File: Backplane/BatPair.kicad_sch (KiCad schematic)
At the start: 6 parts

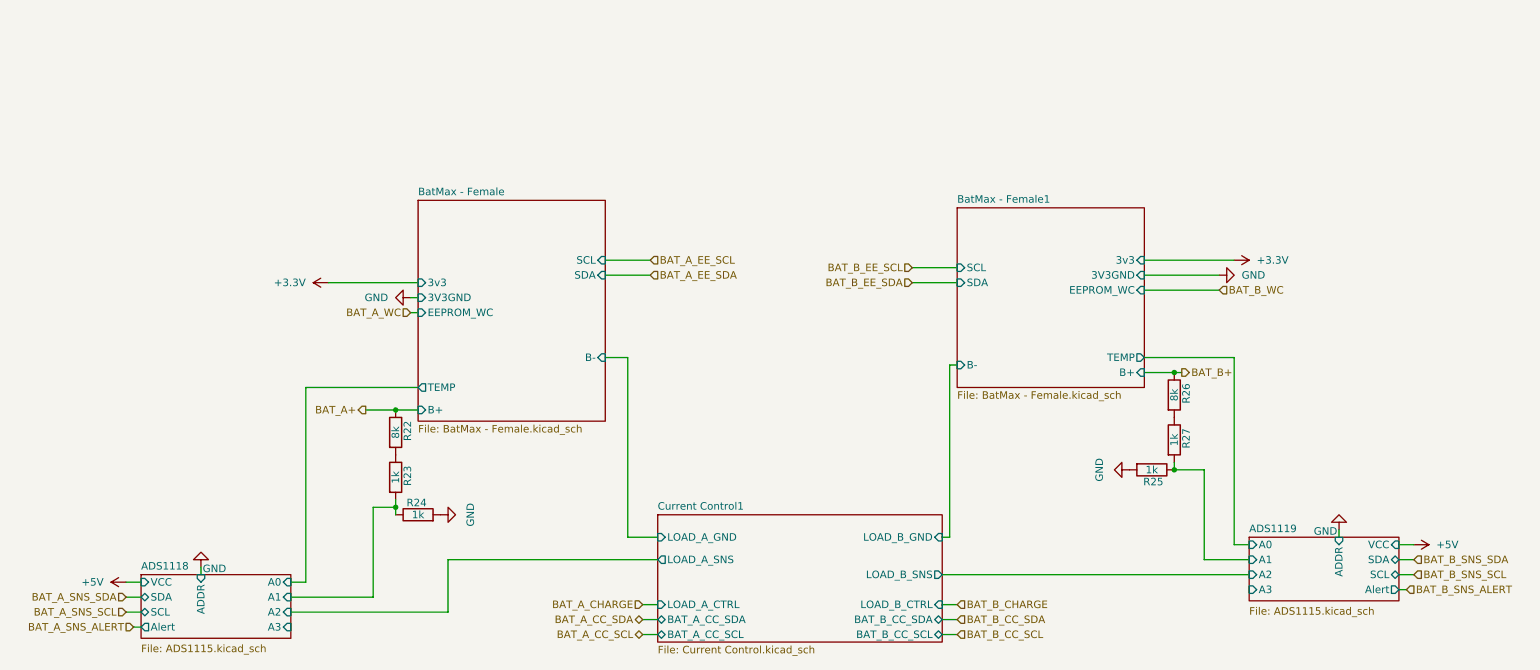
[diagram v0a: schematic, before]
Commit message: added
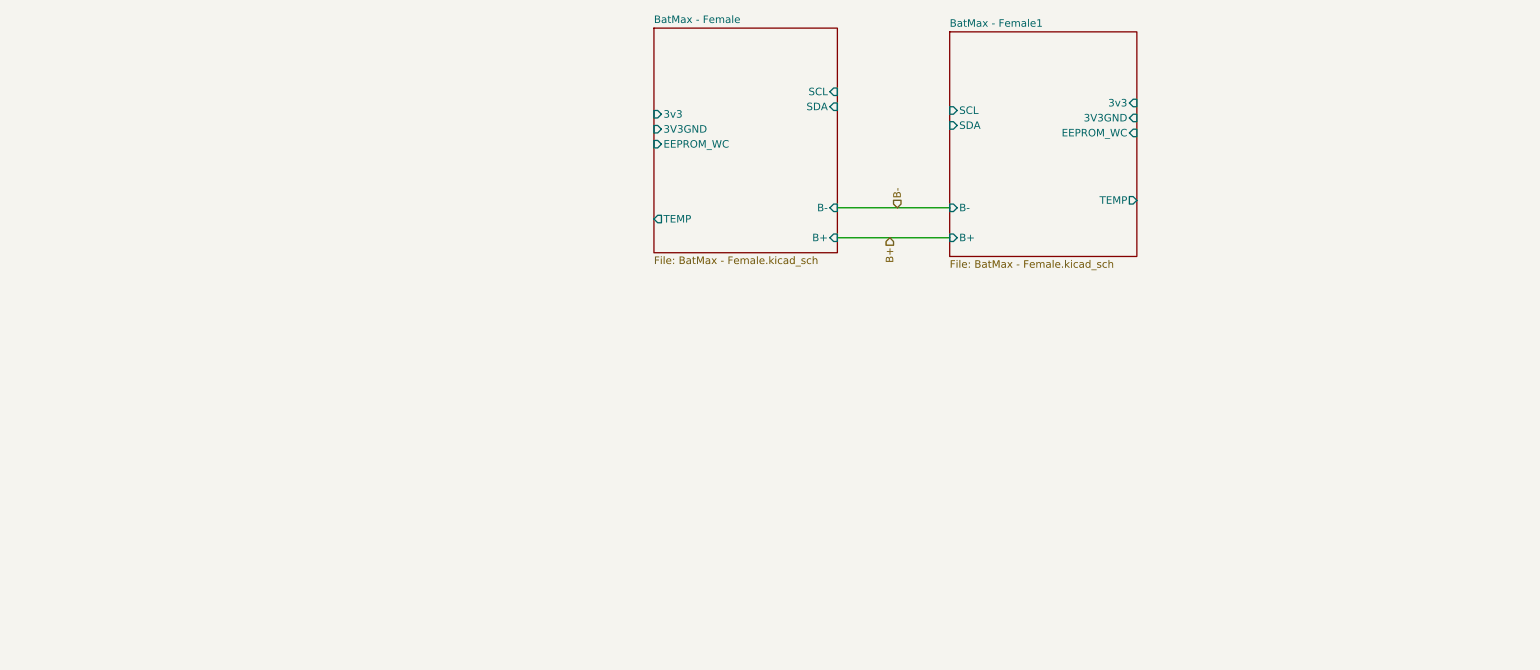
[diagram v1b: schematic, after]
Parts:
- removed R22, R26: 8k, Resistor_SMD:R_1206_3216Metric_Pad1.30x1.75mm_HandSolder, symbol Device:R
- removed R23, R24, R25, R27: 1k, Resistor_SMD:R_1206_3216Metric_Pad1.30x1.75mm_HandSolder, symbol Device:R
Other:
- removed sheet ADS1118
- removed sheet ADS1119
- removed sheet Current Control1
